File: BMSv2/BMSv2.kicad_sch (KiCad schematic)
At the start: 120 parts, among them J2 Conn_01x04_Socket, J3 Conn_01x02_Pin, Q1 AO3401A, SW1 SW_BOOT0, U1 STM32F405RGTx, U2 MCP2561-E-SN, U4 MP2332H, U5 AMS1117-3.3

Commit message: Add files via upload
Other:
- note added: "Balanser"
- note added: "High_speed_clock"
- note added: "Led_status"
- note added: "NTC_Temp_Controll"
- note added: "Overvoltage Protection"
- note added: "Power_connector"
- note added: "Programator"
- note added: "WCS1500_current_sensor"
- moved on the sheet: C13, C14, C15, C16, C17, C18, C19, C20, C21, C22, C23, C24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

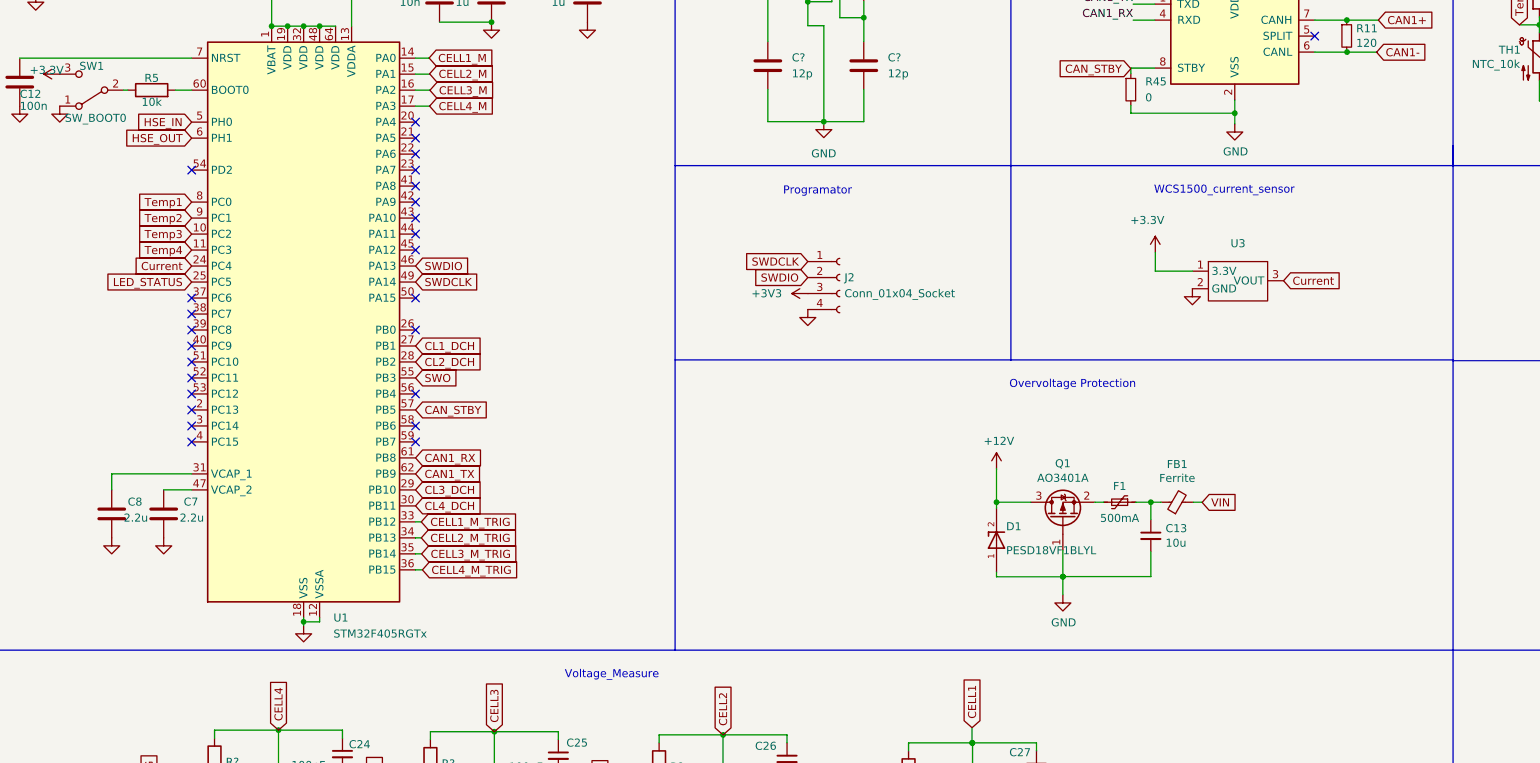
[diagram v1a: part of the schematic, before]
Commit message: Add files via upload
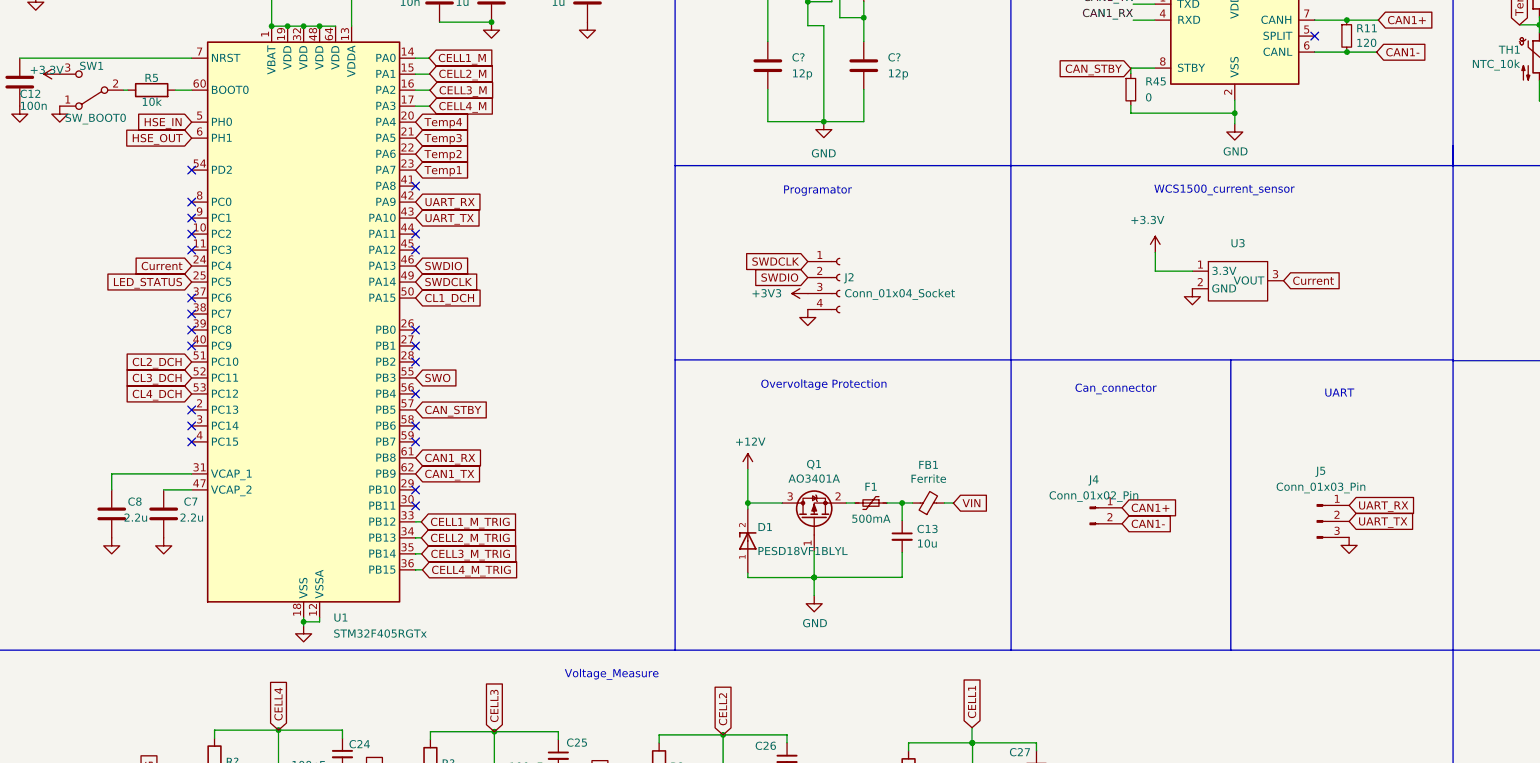
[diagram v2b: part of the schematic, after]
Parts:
- added J4: Conn_01x02_Pin, Connector_Molex:Molex_KK-254_AE-6410-02A_1x02_P2.54mm_Vertical, symbol Connector:Conn_01x02_Pin
- added J5: Conn_01x03_Pin, Connector_PinHeader_2.54mm:PinHeader_1x03_P2.54mm_Vertical, symbol Connector:Conn_01x03_Pin
- J3: footprint Connector_JST:JST_XA_S02B-XASK-1_1x02_P2.50mm_Horizontal -> Connector_Molex:Molex_KK-254_AE-6410-02A_1x02_P2.54mm_Vertical
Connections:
- net CAN1+: now also J4.1 (Pin_1)
- net CAN1-: now also J4.2 (Pin_2)
- net CL1_DCH: now also U1.50 (PA15); no longer U1.27 (PB1)
- net CL2_DCH: now also U1.51 (PC10); no longer U1.28 (PB2)
- net CL3_DCH: now also U1.52 (PC11); no longer U1.29 (PB10)
- net CL4_DCH: now also U1.53 (PC12); no longer U1.30 (PB11)
- net GND: now also J5.3 (Pin_3)
- net Temp1: now also U1.23 (PA7); no longer U1.8 (PC0)
- net Temp2: now also U1.22 (PA6); no longer U1.9 (PC1)
- net Temp3: now also U1.21 (PA5); no longer U1.10 (PC2)
- net Temp4: now also U1.20 (PA4); no longer U1.11 (PC3)
- net UART_RX: now reaches U1.42 (PA9)
- net UART_RX: now also J5.1 (Pin_1)
- net UART_TX: now reaches U1.43 (PA10)
- net UART_TX: now also J5.2 (Pin_2)
- no-connect marks 26 -> 24
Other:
- note added: "Can_connector"
- note added: "UART"
- moved on the sheet: C13, D1, F1, FB1, Q1
